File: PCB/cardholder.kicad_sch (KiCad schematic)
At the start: 2 parts

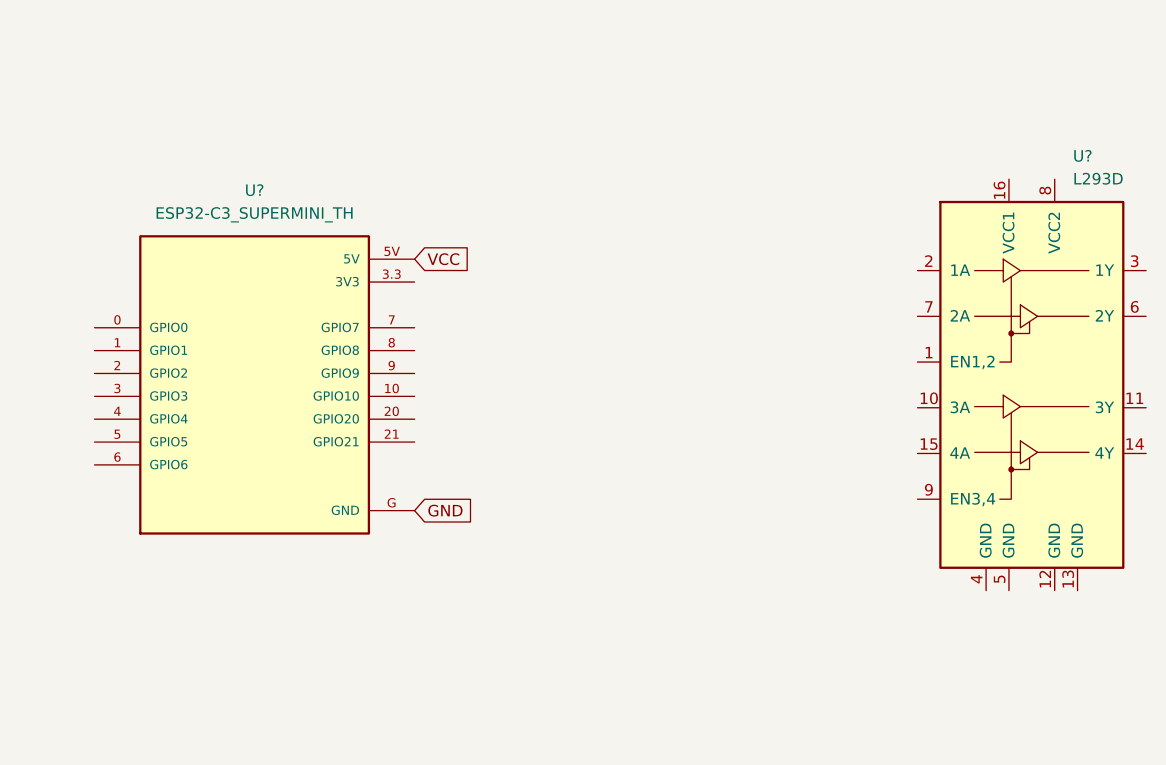
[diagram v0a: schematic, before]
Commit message: main
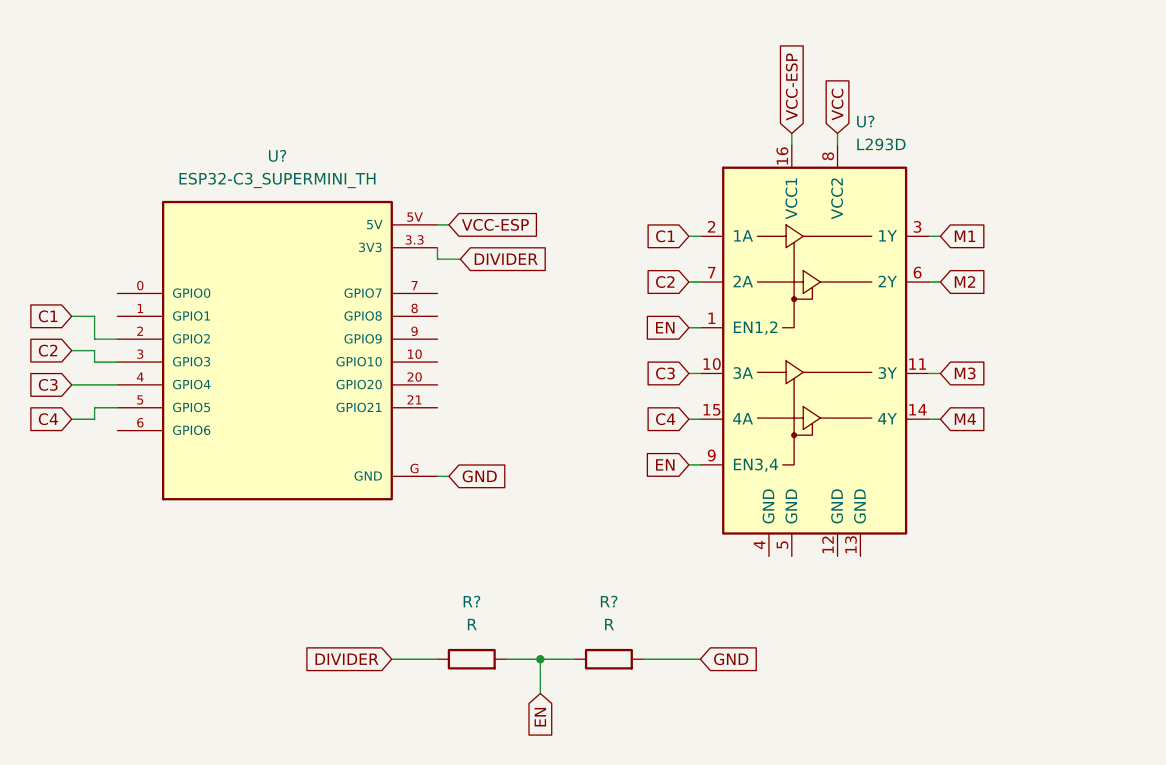
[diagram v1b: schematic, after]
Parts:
- added R? (x2): R, symbol Device:R
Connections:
- net GND: now also R?.2
- net VCC: now also U?.8 (VCC2); no longer U?.5V
- net EN: now reaches U?.1 (EN1,2)
- net EN: now also U?.9 (EN3,4), R?.1, R?.2
- net C3: now reaches U?.10 (3A)
- net C3: now also U?.4 (GPIO4)
- net M3: now reaches U?.11 (3Y)
- net M4: now reaches U?.14 (4Y)
- net C4: now reaches U?.15 (4A)
- net C4: now also U?.5 (GPIO5)
- net VCC-ESP: now reaches U?.16 (VCC1)
- net VCC-ESP: now also U?.5V
- net С1: now reaches U?.2 (1A)
- net M1: now reaches U?.3 (1Y)
- net M2: now reaches U?.6 (2Y)
- net С2: now reaches U?.7 (2A)
- net C1: now reaches U?.2 (GPIO2)
- net C2: now reaches U?.3 (GPIO3)
- net DIVIDER: now reaches U?.3.3 (3V3)
- net DIVIDER: now also R?.1
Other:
- moved on the sheet: U?
